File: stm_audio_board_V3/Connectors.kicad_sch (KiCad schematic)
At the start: 9 parts, among them J1 Power conn, J2 STlink, J3 Audio_sig, J4 Conn_01x01_taptempo, J6 Conn_01x03_pot_ext

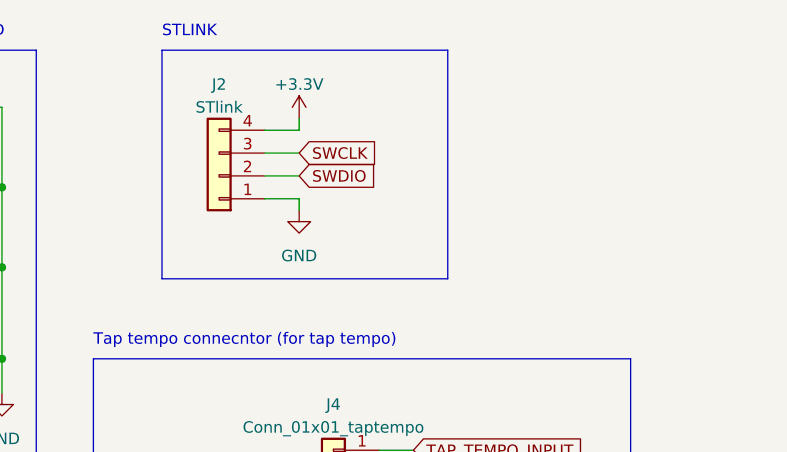
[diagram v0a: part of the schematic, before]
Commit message: minor changes
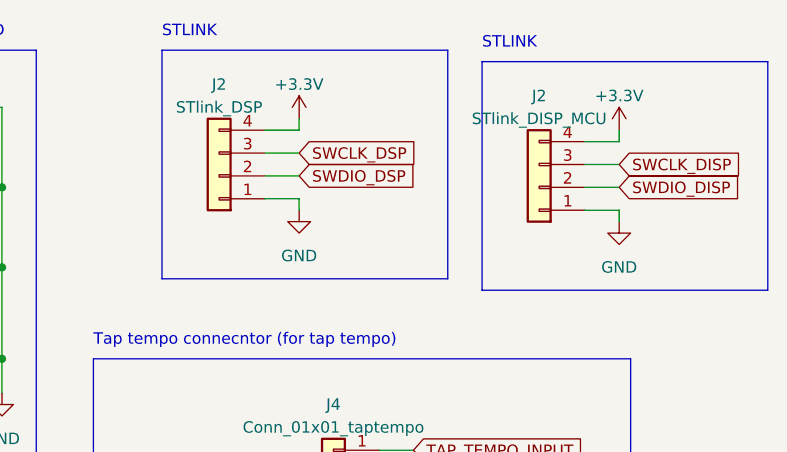
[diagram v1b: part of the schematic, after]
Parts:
- added J2: STlink_DISP_MCU, Connector_PinHeader_2.54mm:PinHeader_1x04_P2.54mm_Vertical, symbol Connector_Generic:Conn_01x04
- J2: value STlink -> STlink_DSP
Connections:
- net +3.3V: now also J2.4 (Pin_4)
- net GND: now also J2.1 (Pin_1)
- net SWCLK renamed SWCLK_DSP
- net SWDIO renamed SWDIO_DSP
- new net SWCLK_DISP: J2.3 (Pin_3)
- new net SWDIO_DISP: J2.2 (Pin_2)
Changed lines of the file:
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@@
+    (stroke (width 0) (type default))
+  )
+  (wire (pts (xy 177.8 34.29) (xy 181.61 34.29))
     (stroke (width 0) (type default))
   )
@@
     (stroke (width 0) (type default))
   )
+  (wire (pts (xy 181.61 43.18) (xy 181.61 41.91))
+    (stroke (width 0) (type default))
+  )
+  (wire (pts (xy 181.61 41.91) (xy 177.8 41.91))
+    (stroke (width 0) (type default))
+  )
+  (wire (pts (xy 177.8 36.83) (xy 181.61 36.83))
+    (stroke (width 0) (type default))
+  )
   (wire (pts (xy 146.05 41.91) (xy 146.05 40.64))
     (stroke (width 0) (type default))
@@
     (stroke (width 0) (type default))
   )
+  (wire (pts (xy 177.8 39.37) (xy 181.61 39.37))
+    (stroke (width 0) (type default))
+  )
   (wire (pts (xy 49.53 57.15) (xy 52.07 57.15))
     (stroke (width 0) (type default))
@@
     (stroke (width 0) (type default))
   )
+  (wire (pts (xy 181.61 33.02) (xy 181.61 34.29))
+    (stroke (width 0) (type default))
+  )
   (wire (pts (xy 105.41 39.37) (xy 113.03 39.37))
     (stroke (width 0) (type default))
@@
   )
   (rectangle (start 27.94 135.89) (end 81.28 156.21)
+    (stroke (width 0) (type default))
+    (fill (type none))
+  )
+  (rectangle (start 166.37 25.4) (end 198.12 50.8)
     (stroke (width 0) (type default))
     (fill (type none))
@@
     (effects (font (size 1.27 1.27)) (justify left bottom))
   )
+  (text "STLINK" (at 166.37 24.13 0)
+    (effects (font (size 1.27 1.27)) (justify left bottom))
+  )
   (text "External potentiometer\n" (at 27.94 134.62 0)
     (effects (font (size 1.27 1.27)) (justify left bottom))
@@
     )
   )
-  (global_label "SWCLK" (shape input) (at 146.05 35.56 0) (fields_autoplaced)
-    (effects (font (size 1.27 1.27)) (justify left))
-    (property "Intersheetrefs" "${INTERSHEET_REFS}" (at 155.1848 35.56 0)
+  (global_label "SWCLK_DSP" (shape input) (at 146.05 35.56 0) (fields_autoplaced)
+    (effects (font (size 1.27 1.27)) (justify left))
+    (property "Intersheetrefs" "${INTERSHEET_REFS}" (at 159.9019 35.56 0)
       (effects (font (size 1.27 1.27)) (justify left) hide)
     )
@@
     )
   )
+  (global_label "SWCLK_DISP" (shape input) (at 181.61 36.83 0) (fields_autoplaced)
+    (effects (font (size 1.27 1.27)) (justify left))
+    (property "Intersheetrefs" "${INTERSHEET_REFS}" (at 196.0667 36.83 0)
+      (effects (font (size 1.27 1.27)) (justify left) hide)
+    )
+  )
+  (global_label "SWDIO_DISP" (shape input) (at 181.61 39.37 0) (fields_autoplaced)
+    (effects (font (size 1.27 1.27)) (justify left))
+    (property "Intersheetrefs" "${INTERSHEET_REFS}" (at 195.7039 39.37 0)
+      (effects (font (size 1.27 1.27)) (justify left) hide)
+    )
+  )
   (global_label "PWR_INPUT_12V-18V" (shape input) (at 53.34 81.28 0) (fields_autoplaced)
     (effects (font (size 1.27 1.27)) (justify left))
@@
     )
   )
-  (global_label "SWDIO" (shape input) (at 146.05 38.1 0) (fields_autoplaced)
-    (effects (font (size 1.27 1.27)) (justify left))
-    (property "Intersheetrefs" "${INTERSHEET_REFS}" (at 154.822 38.1 0)
+  (global_label "SWDIO_DSP" (shape input) (at 146.05 38.1 0) (fields_autoplaced)
+    (effects (font (size 1.27 1.27)) (justify left))
+    (property "Intersheetrefs" "${INTERSHEET_REFS}" (at 159.5391 38.1 0)
       (effects (font (size 1.27 1.27)) (justify left) hide)
     )
@@
       (effects (font (size 1.27 1.27)))
     )
-    (property "Value" "STlink" (at 137.16 30.48 0)
+    (property "Value" "STlink_DSP" (at 137.16 30.48 0)
       (effects (font (size 1.27 1.27)))
     )
@@
     )
   )
+  (symbol (lib_id "power:GND") (at 181.61 43.18 0) (unit 1)
+    (in_bom yes) (on_board yes) (dnp no) (fields_autoplaced)
+    (property "Reference" "#PWR011" (at 181.61 49.53 0)
+      (effects (font (size 1.27 1.27)) hide)
+    )
+    (property "Value" "GND" (at 181.61 48.26 0)
+      (effects (font (size 1.27 1.27)))
+    )
+    (property "Footprint" "" (at 181.61 43.18 0)
+      (effects (font (size 1.27 1.27)) hide)
+    )
+    (property "Datasheet" "" (at 181.61 43.18 0)
+      (effects (font (size 1.27 1.27)) hide)
+    )
+    (pin "1")
+    (instances
+      (project "stm_audio_board_V3"
+        (path "/6997cf63-2615-4e49-9471-e7da1b6bae71"
+          (reference "#PWR011") (unit 1)
+        )
+        (path "/6997cf63-2615-4e49-9471-e7da1b6bae71/51aec99e-3301-49b6-8e7f-31ba63a05d64"
+          (reference "#PWR011") (unit 1)
+        )
+        (path "/6997cf63-2615-4e49-9471-e7da1b6bae71/6424856c-1346-4018-a943-0d16008c9545"
+          (reference "#PWR0109") (unit 1)
+        )
+      )
+    )
+  )
   (symbol (lib_id "power:+3.3V") (at 146.05 31.75 0) (unit 1)
     (in_bom yes) (on_board yes) (dnp no) (fields_autoplaced)
@@
         )
       )
+    )
+  )
+  (symbol (lib_id "Connector_Generic:Conn_01x04") (at 172.72 39.37 180) (unit 1)
+    (in_bom yes) (on_board yes) (dnp no) (fields_autoplaced)
+    (property "Reference" "J2" (at 172.72 29.21 0)
+      (effects (font (size 1.27 1.27)))
+    )
+    (property "Value" "STlink_DISP_MCU" (at 172.72 31.75 0)
+      (effects (font (size 1.27 1.27)))
+    )
+    (property "Footprint" "Connector_PinHeader_2.54mm:PinHeader_1x04_P2.54mm_Vertical" (at 172.72 39.37 0)
+      (effects (font (size 1.27 1.27)) hide)
+    )
+    (property "Datasheet" "~" (at 172.72 39.37 0)
+      (effects (font (size 1.27 1.27)) hide)
+    )
+    (pin "1")
+    (pin "2")
+    (pin "3")
+    (pin "4")
+    (instances
+      (project "stm_audio_board_V3"
+        (path "/6997cf63-2615-4e49-9471-e7da1b6bae71"
+          (reference "J2") (unit 1)
+        )
+        (path "/6997cf63-2615-4e49-9471-e7da1b6bae71/51aec99e-3301-49b6-8e7f-31ba63a05d64"
+          (reference "J2") (unit 1)
+        )
+        (path "/6997cf63-2615-4e49-9471-e7da1b6bae71/6424856c-1346-4018-a943-0d16008c9545"
+          (reference "J16") (unit 1)
+        )
+      )
+    )
+  )
+  (symbol (lib_id "power:+3.3V") (at 181.61 33.02 0) (unit 1)
+    (in_bom yes) (on_board yes) (dnp no) (fields_autoplaced)
+    (property "Reference" "#PWR0108" (at 181.61 36.83 0)
+      (effects (font (size 1.27 1.27)) hide)
+    )
+    (property "Value" "+3.3V" (at 181.61 29.21 0)
+      (effects (font (size 1.27 1.27)))
+    )
+    (property "Footprint" "" (at 181.61 33.02 0)
+      (effects (font (size 1.27 1.27)) hide)
+    )
+    (property "Datasheet" "" (at 181.61 33.02 0)
+      (effects (font (size 1.27 1.27)) hide)
+    )
+    (pin "1")
+    (instances
+      (project "stm_audio_board_V3"
+        (path "/6997cf63-2615-4e49-9471-e7da1b6bae71/6424856c-1346-4018-a943-0d16008c9545"
+          (reference "#PWR0108") (unit 1)
+        )
+      )

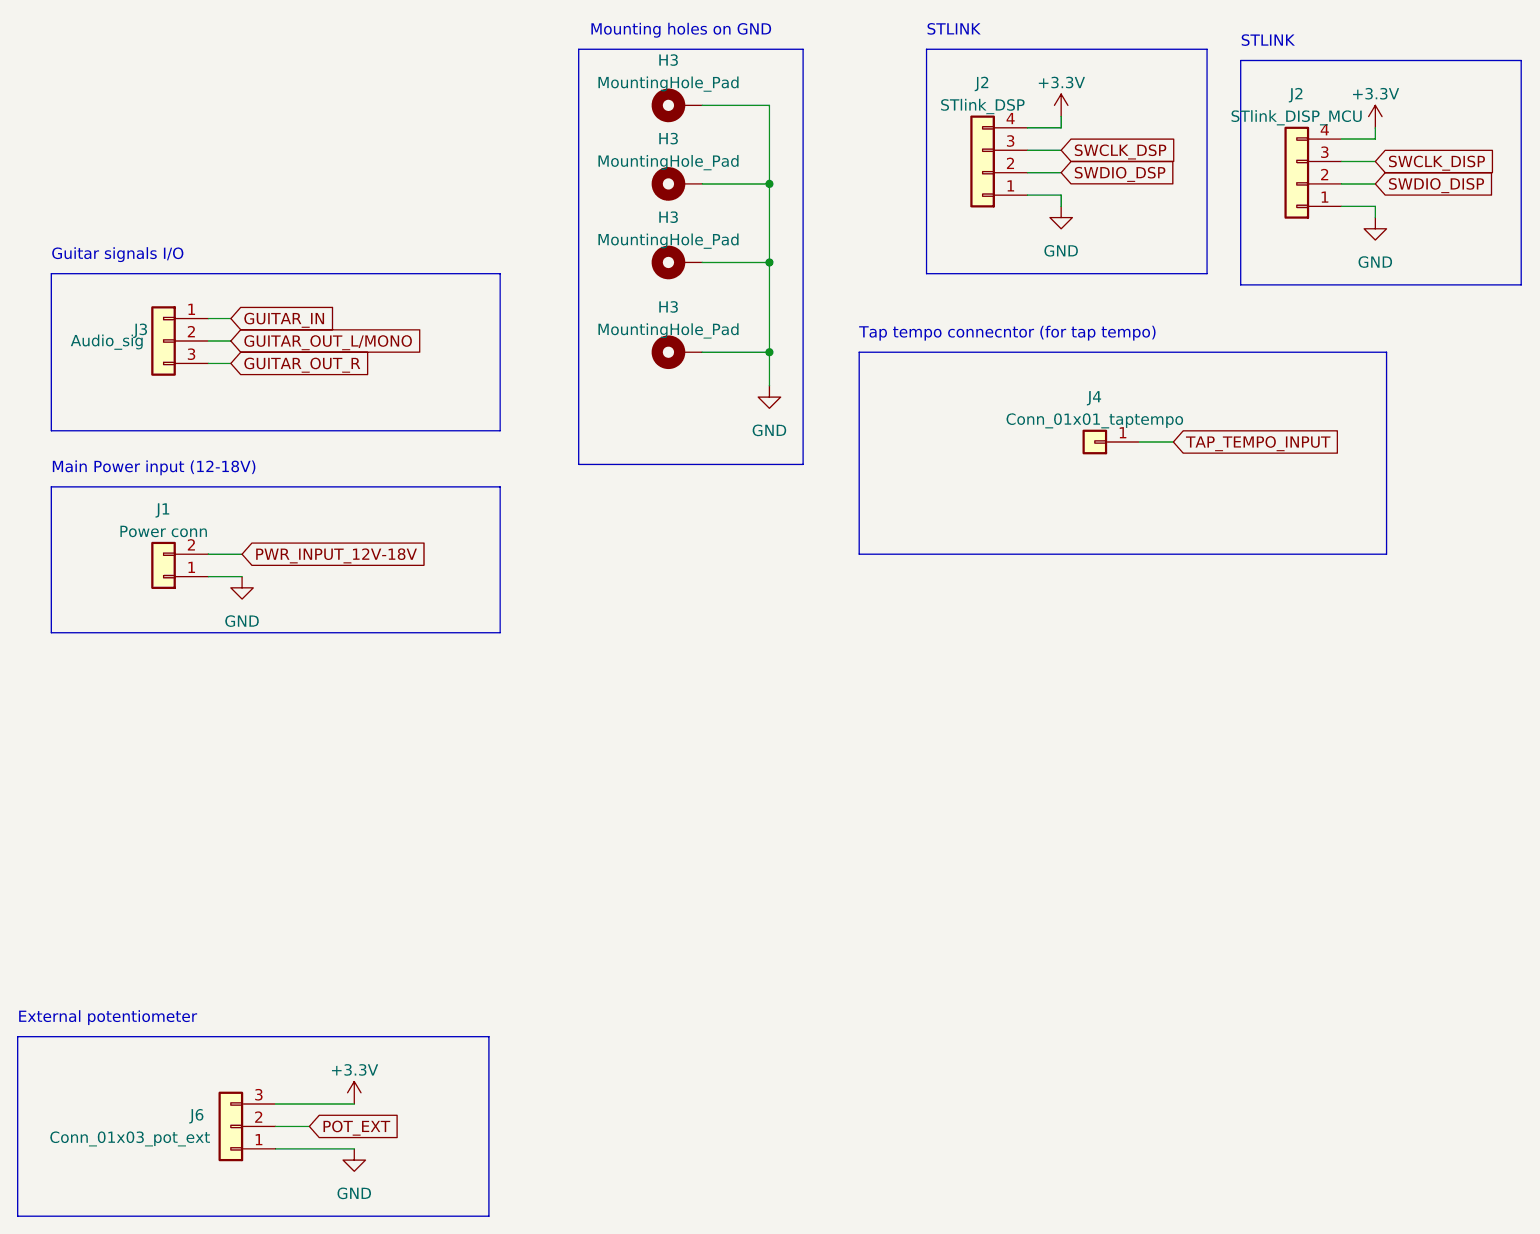
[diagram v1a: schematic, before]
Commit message: minor commit
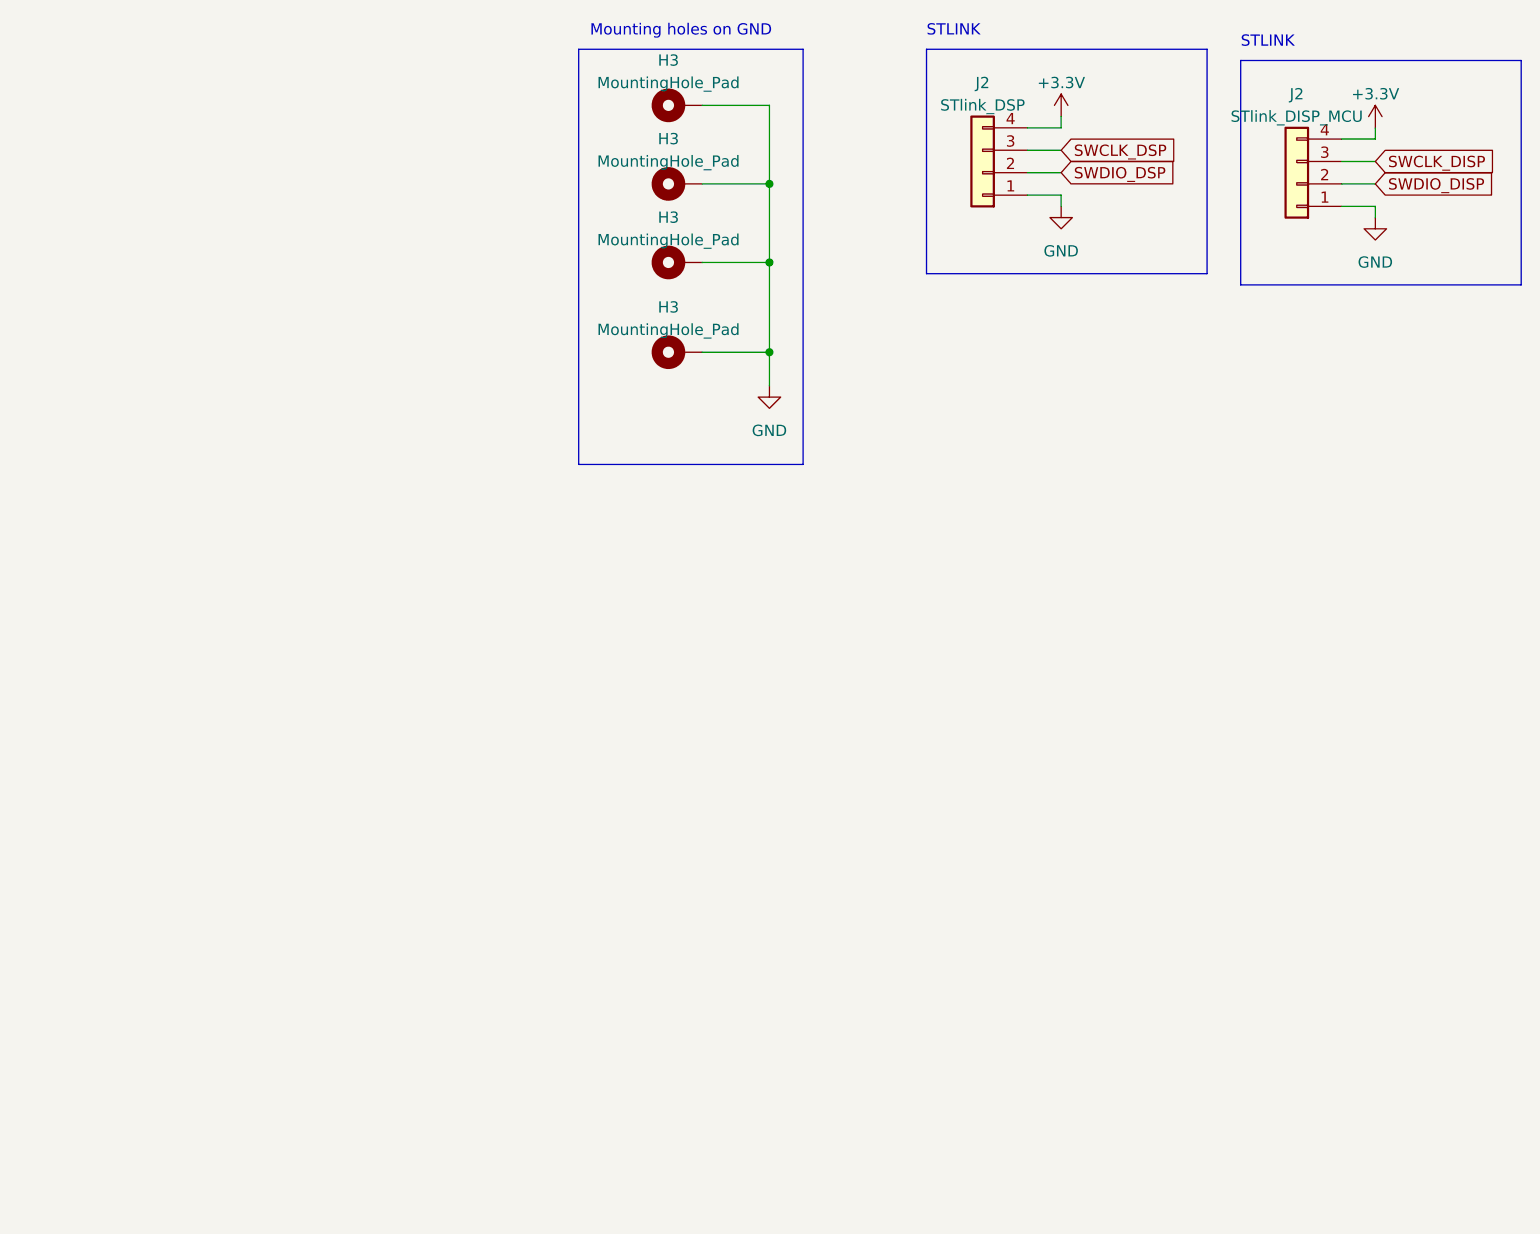
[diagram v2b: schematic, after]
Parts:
- removed J1: Power conn, Connector_PinHeader_2.54mm:PinHeader_1x02_P2.54mm_Vertical, symbol Connector_Generic:Conn_01x02
- removed J3: Audio_sig, Connector_PinHeader_2.54mm:PinHeader_1x03_P2.54mm_Vertical, symbol Connector_Generic:Conn_01x03
- removed J4: Conn_01x01_taptempo, Connector_PinHeader_2.54mm:PinHeader_1x01_P2.54mm_Vertical, symbol Connector_Generic:Conn_01x01
- removed J6: Conn_01x03_pot_ext, Connector_PinHeader_2.54mm:PinHeader_1x03_P2.54mm_Vertical, symbol Connector_Generic:Conn_01x03
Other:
- note removed: "External potentiometer"
- note removed: "Guitar signals I/O"
- note removed: "Main Power input (12-18V)"
- note removed: "Tap tempo connecntor (for tap tempo)"
